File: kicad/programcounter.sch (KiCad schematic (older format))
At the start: 6 parts, among them U13 74LS161, U14 74LS245

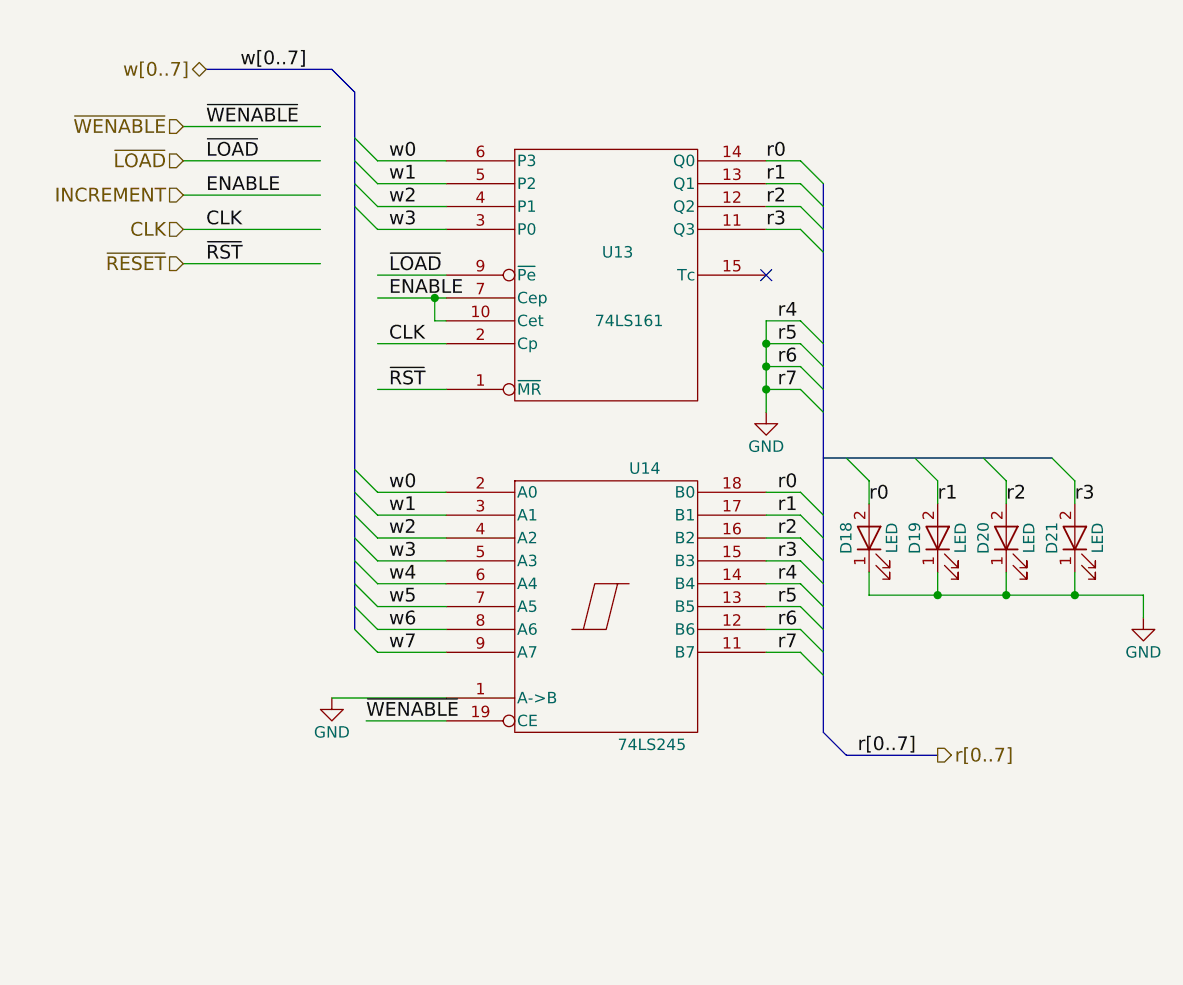
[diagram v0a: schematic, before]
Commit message: Update to current kicad libraries
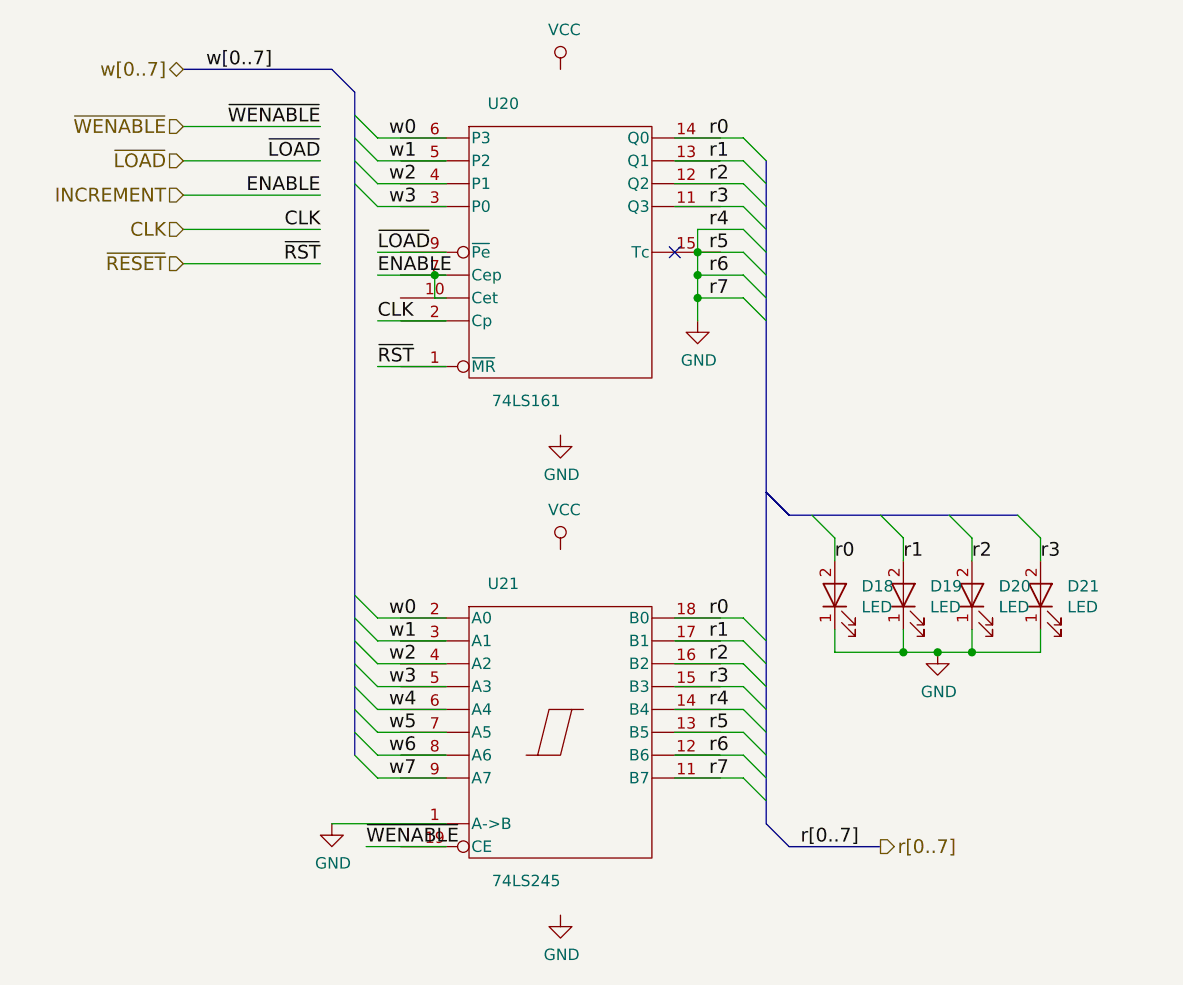
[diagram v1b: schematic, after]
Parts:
- removed D18, D19, D20, D21: LED, LEDs:LED-5MM, symbol LED
- removed U13: 74LS161, Housings_DIP:DIP-16_W7.62mm_LongPads, symbol 74LS161
- removed U14: 74LS245, Housings_DIP:DIP-20_W7.62mm_LongPads, symbol 74LS245
- added D18, D19, D20, D21: LED, symbol Device:LED
- added U20: 74LS161, symbol 74xx:74LS161
- added U21: 74LS245, symbol 74xx:74LS245
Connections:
- net labels added: VCC
- wire segments 52 -> 58
